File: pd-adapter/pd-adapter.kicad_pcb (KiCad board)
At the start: 4 copper layers, 45 x 38 mm, 59 parts, among them J1 USB, J2 DBG, J3 EXT, SW1 RST, SW2 USER, U1 FUSB302BMPX, U2 TPS54202DDC, U3 STM32F072C8Tx

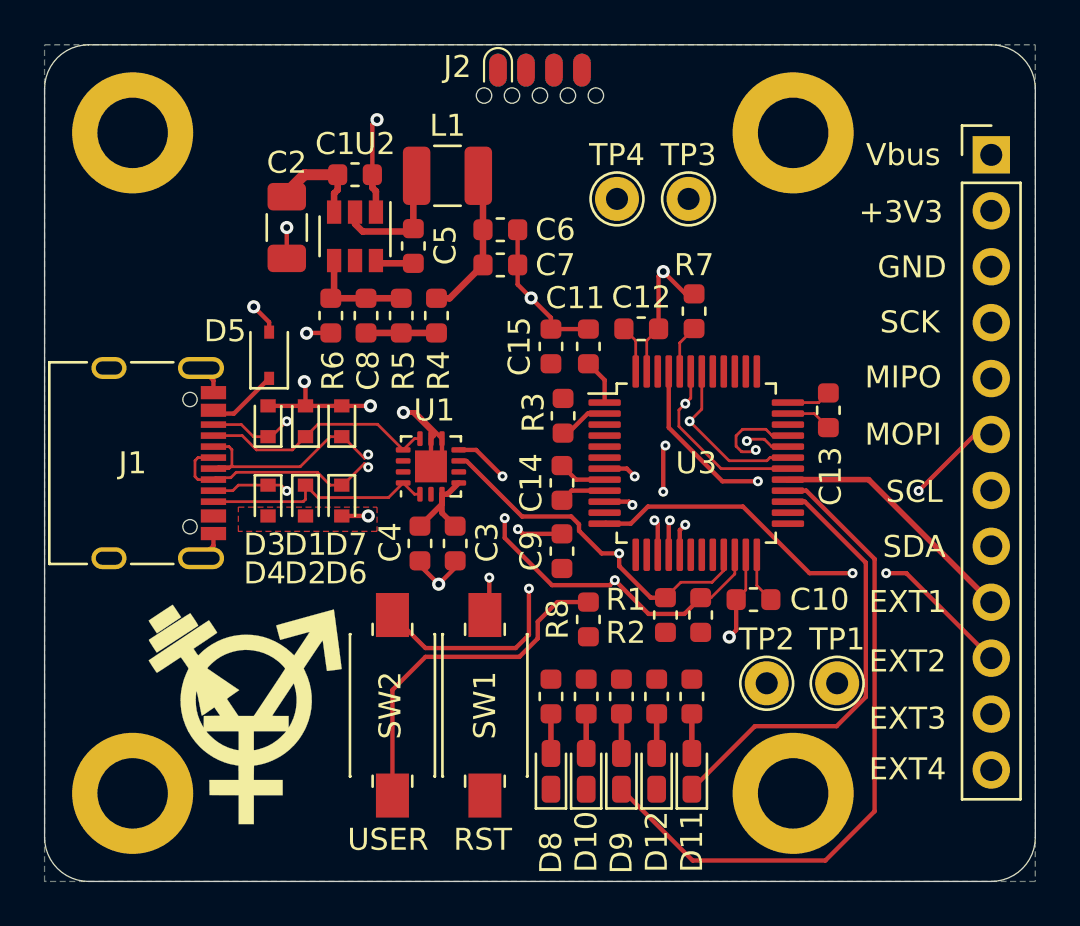
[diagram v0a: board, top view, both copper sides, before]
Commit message: First pass at adapter layout, needs second revision
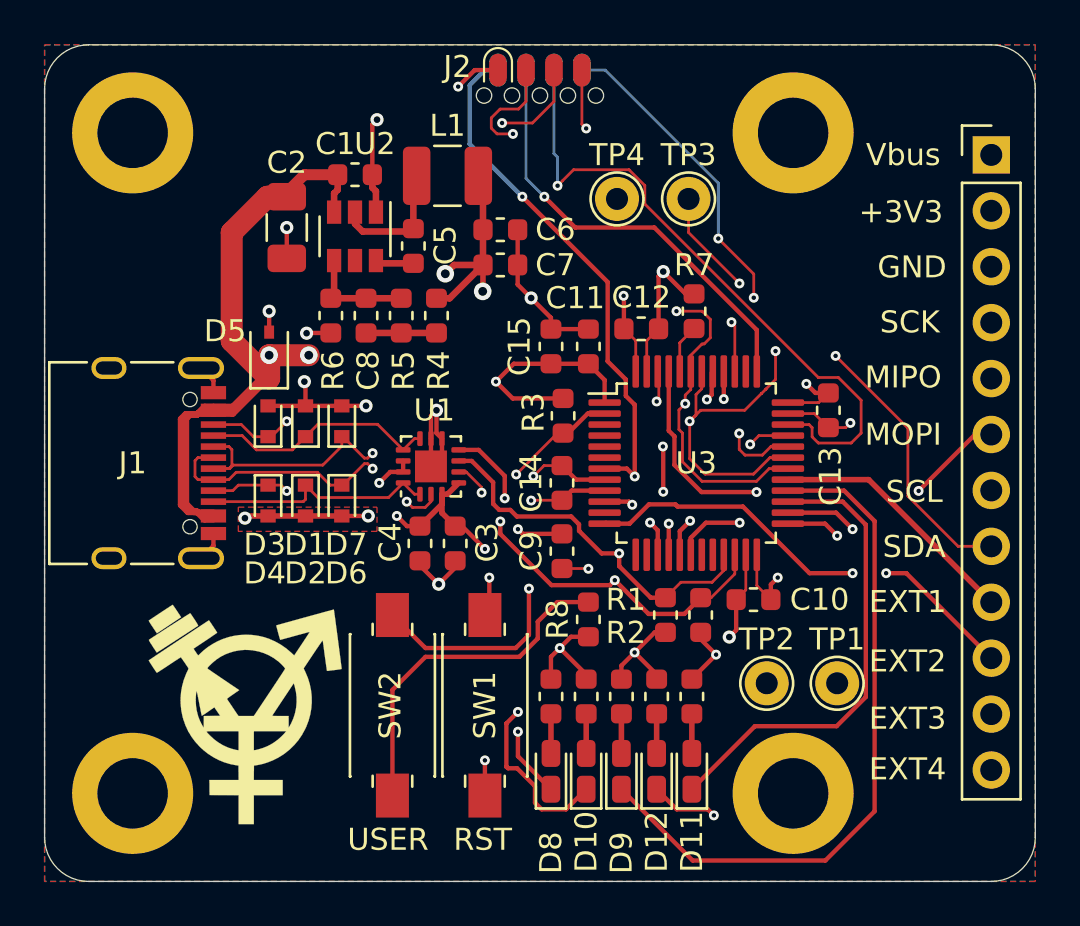
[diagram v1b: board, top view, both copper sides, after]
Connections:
- U3 pad 13: /EXT_3 -> Net-(U3-Pad13)
- U3 pad 14: /EXT_4 -> Net-(U3-Pad14)
- U3 pad 25: Net-(U3-Pad25) -> /EXT_4
- U3 pad 26: Net-(U3-Pad26) -> /EXT_3
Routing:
- net +3V3: track 22.1 -> 58.0 mm, vias 0 -> 14
- net VBUS: track 7.80 -> 40.5 mm, vias 0 -> 3
- net /SWDIO: track 0.00 -> 29.8 mm, vias 0 -> 1
- net /LED_GRN: track 0.00 -> 27.1 mm, vias 0 -> 2
- net /D-: track 30.4 -> 54.1 mm, vias 2 -> 3
- net /LED_RED: track 0.00 -> 23.5 mm, vias 0 -> 2
- net /SDA_EXT: track 0.00 -> 22.9 mm, vias 0 -> 2
- net /~RST: track 14.4 -> 36.9 mm, vias 3 -> 4
- net /D+: track 32.4 -> 53.2 mm, vias 2 -> 3
- net /LED_YLL: track 0.00 -> 20.2 mm, vias 0 -> 2
- net /SWCLK: track 0.00 -> 20.1 mm, vias 0 -> 1
- net /SWO: track 0.00 -> 18.0 mm, vias 0 -> 3
- net /EXT_4: track 0.00 -> 17.1 mm, vias 0 -> 1
- net /EXT_3: track 0.00 -> 15.5 mm, vias 0 -> 1
- net /SBU1: track 32.3 -> 47.4 mm, vias 2 -> 4
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- added copper zone on In2.Cu, net +3V3
- added copper zone on In1.Cu, net VBUS
